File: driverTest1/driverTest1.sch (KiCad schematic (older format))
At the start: 35 parts, among them J1 LED_OUT, J2 INPUT, U1 TPS63020, U2 MCP602, U3 XC6206P332MR

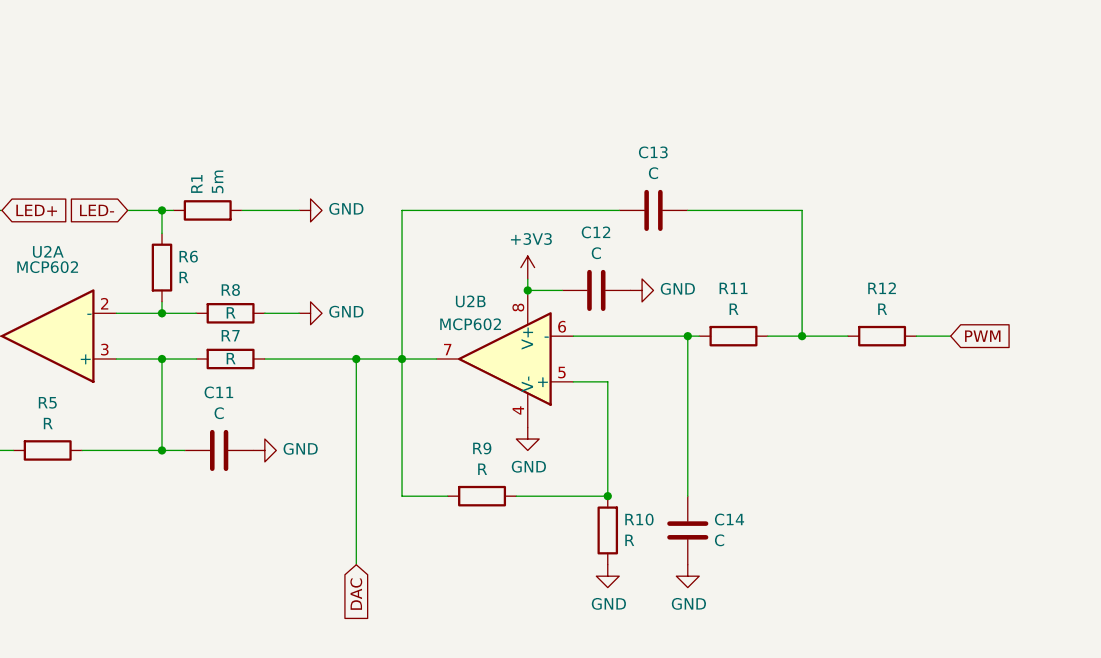
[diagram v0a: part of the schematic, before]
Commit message: Add routing note
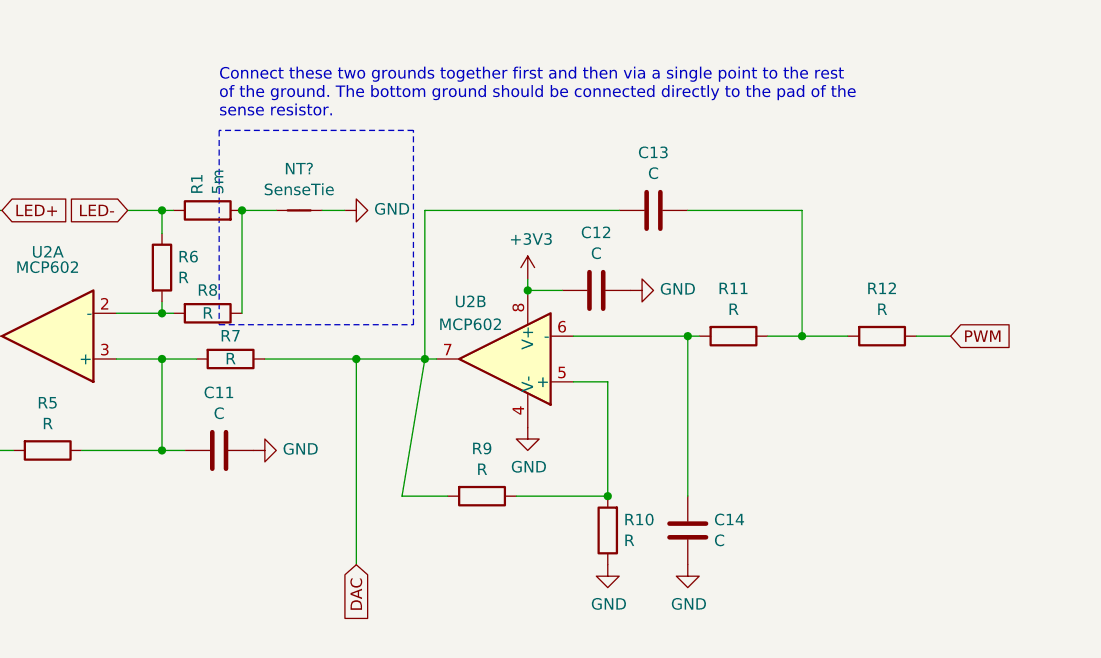
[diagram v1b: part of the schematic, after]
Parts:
- added NT?: SenseTie, NetTie:NetTie-2_SMD_Pad0.5mm, symbol Device:Net-Tie_2
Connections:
- net GND: now also NT?.2; no longer R1.2, R8.1
- new net: NT?.1, R1.2, R8.1
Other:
- note added: "Connect these two grounds together first and then via a single point to the rest\nof the ground. The bottom ground should be connected directly to the pad of the\nsense resistor."
- moved on the sheet: R8
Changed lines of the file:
@@
 L power:GND #PWR0105
 U 1 1 5F1D53F5
-P 7850 1950
-F 0 "#PWR0105" H 7850 1700 50  0001 C CNN
-F 1 "GND" V 7855 1822 50  0000 R CNN
-F 2 "" H 7850 1950 50  0001 C CNN
-F 3 "" H 7850 1950 50  0001 C CNN
-	1    7850 1950
+P 8050 1950
+F 0 "#PWR0105" H 8050 1700 50  0001 C CNN
+F 1 "GND" V 8055 1822 50  0000 R CNN
+F 2 "" H 8050 1950 50  0001 C CNN
+F 3 "" H 8050 1950 50  0001 C CNN
+	1    8050 1950
 	0    -1   -1   0
 $EndComp
@@
 L Device:R R8
 U 1 1 5F1D8F6D
-P 7550 2400
-F 0 "R8" V 7450 2400 50  0000 C CNN
-F 1 "R" V 7550 2400 50  0000 C CNN
-F 2 "Resistor_SMD:R_0603_1608Metric" V 7480 2400 50  0001 C CNN
-F 3 "~" H 7550 2400 50  0001 C CNN
-	1    7550 2400
+P 7450 2400
+F 0 "R8" V 7350 2400 50  0000 C CNN
+F 1 "R" V 7450 2400 50  0000 C CNN
+F 2 "Resistor_SMD:R_0603_1608Metric" V 7380 2400 50  0001 C CNN
+F 3 "~" H 7450 2400 50  0001 C CNN
+	1    7450 2400
 	0    1    1    0
 $EndComp
@@
 	7250 1950 7100 1950
 Wire Wire Line
-	7400 2400 7250 2400
+	7300 2400 7250 2400
 Wire Wire Line
 	7250 2400 7250 2350
@@
 	8500 3200 8300 3200
 Wire Wire Line
-	8300 3200 8300 2600
-Wire Wire Line
-	8300 2600 8450 2600
+	8300 3200 8400 2600
+Wire Wire Line
+	8400 2600 8450 2600
 $Comp
 L Amplifier_Operational:MCP602 U2
@@
 	10050 1950 9550 1950
 Wire Wire Line
-	9250 1950 8300 1950
-Wire Wire Line
-	8300 1950 8300 2600
-Connection ~ 8300 2600
-Wire Wire Line
-	8300 2600 8100 2600
+	9250 1950 8400 1950
+Wire Wire Line
+	8400 1950 8400 2600
+Connection ~ 8400 2600
+Wire Wire Line
+	8400 2600 8100 2600
 Wire Wire Line
 	8100 2600 8100 3500
@@
 Text GLabel 2750 6050 2    50   Input ~ 0
 DAC
-Wire Wire Line
-	7600 1950 7850 1950
-$Comp
-L power:GND #PWR0131
-U 1 1 5F329A72
-P 7850 2400
-F 0 "#PWR0131" H 7850 2150 50  0001 C CNN
-F 1 "GND" V 7855 2272 50  0000 R CNN
-F 2 "" H 7850 2400 50  0001 C CNN
-F 3 "" H 7850 2400 50  0001 C CNN
-	1    7850 2400
-	0    -1   -1   0
-$EndComp
-Wire Wire Line
-	7850 2400 7700 2400
 $Comp
 L Connector:TestPoint TP1
@@
 Wire Wire Line
 	6300 2350 6300 2500
+Text Notes 7500 1550 0    50   ~ 0
+Connect these two grounds together first and then via a single point to the rest\nof the ground. The bottom ground should be connected directly to the pad of the\nsense resistor.
+$Comp
+L Device:Net-Tie_2 NT?
+U 1 1 5F3732B0
+P 7850 1950
+F 0 "NT?" H 7850 2131 50  0000 C CNN
+F 1 "SenseTie" H 7850 2040 50  0000 C CNN
+F 2 "NetTie:NetTie-2_SMD_Pad0.5mm" H 7850 1950 50  0001 C CNN
+F 3 "~" H 7850 1950 50  0001 C CNN
+	1    7850 1950
+	1    0    0    -1
+$EndComp
+Wire Wire Line
+	7600 2400 7600 1950
+Connection ~ 7600 1950
+Wire Wire Line
+	7600 1950 7750 1950
+Wire Wire Line
+	8050 1950 7950 1950
+Wire Notes Line
+	7500 2450 8350 2450
+Wire Notes Line
+	8350 2450 8350 1600
+Wire Notes Line
+	8350 1600 7500 1600
+Wire Notes Line
+	7500 1600 7500 2450
 $EndSCHEMATC
